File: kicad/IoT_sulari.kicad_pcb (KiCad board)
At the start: 4 copper layers, 50 x 41 mm, 44 parts, among them J1 73412-0110, J2 73412-0110, J20 694106106102, J3 20021121-00010C4LF, J4 20021121-00010C4LF, J40 693043020611, J6 20021121-00010C4LF, SW1 SW_SPST, SW2 TL3301DF160QG, SW3 TL3301DF160QG, SW4 TL3301DF160QG, SW5 TL3301DF160QG, U2 NRF9160, U20 MIC5219-3.3YM5-TR, U40 TPD3F303DPVR

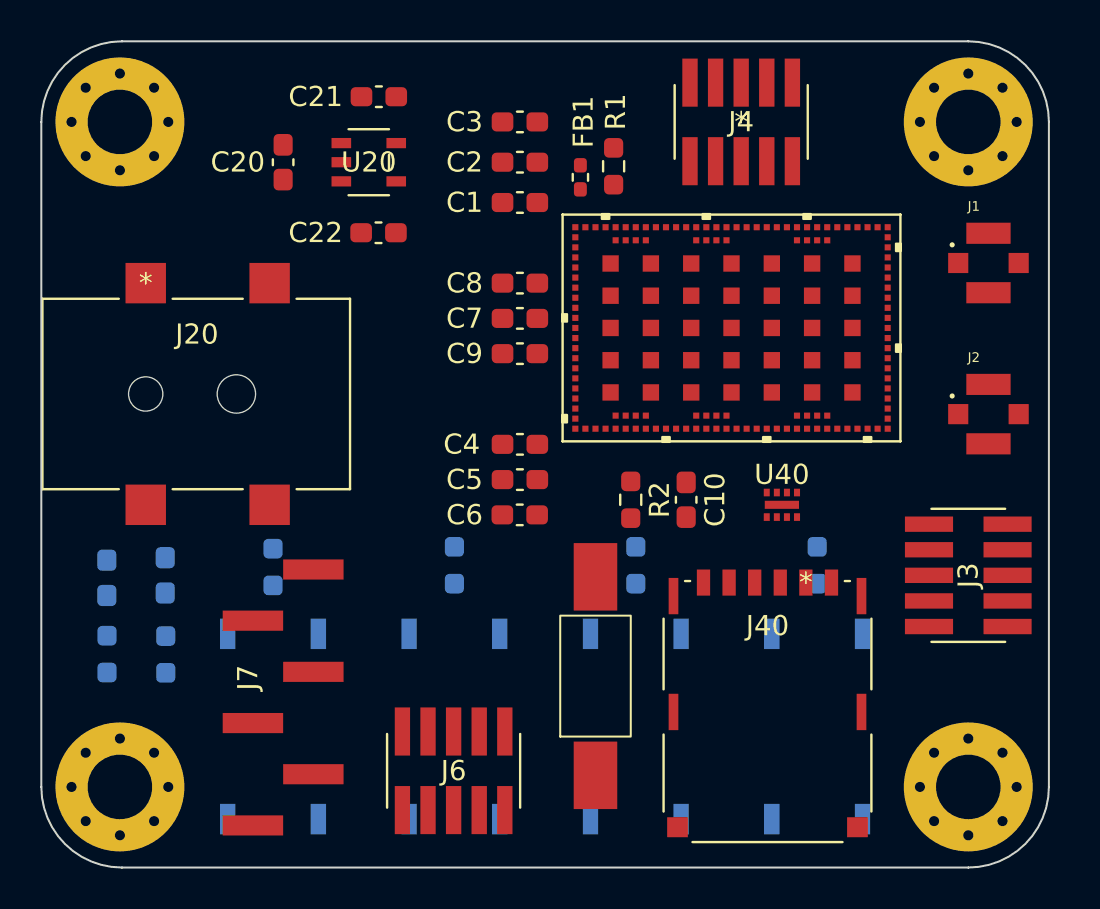
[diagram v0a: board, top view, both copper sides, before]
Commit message: routing
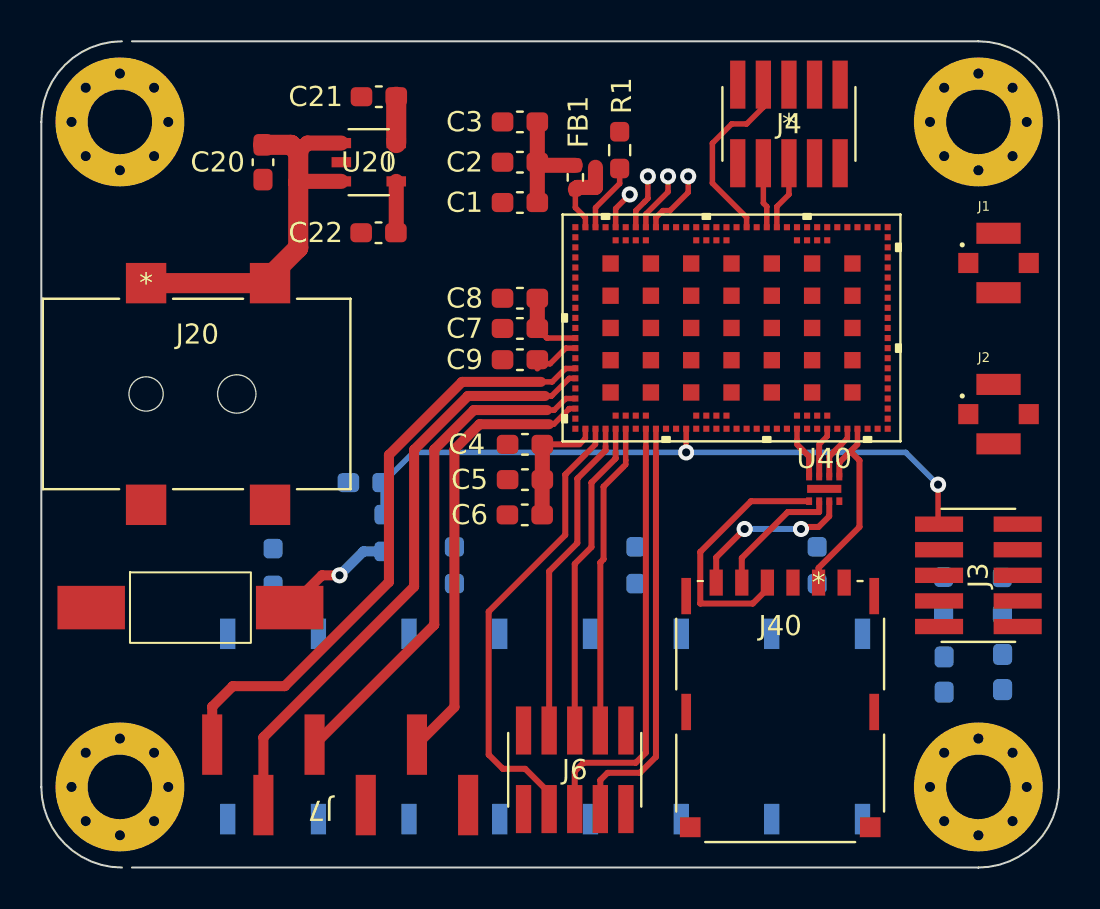
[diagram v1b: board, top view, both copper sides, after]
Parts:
- C10, R2: moved to B.Cu
- moved D2 44.7 mm to (140.2, 66.3), turned to -90 degrees
- moved R4 44.5 mm to (140.2, 62.5), turned to 90 degrees
- moved D1 39.0 mm to (137.3, 66.4), turned to -90 degrees
- moved R3 38.7 mm to (137.3, 62.5), turned to 90 degrees
- moved SW1 20.4 mm to (99.9, 63.1), turned to 0 degrees
- moved C10 15.9 mm to (108.6, 56.9), turned to 180 degrees
- moved R2 12.4 mm to (109.5, 59.4)
- moved J6 6.01 mm to (119.0, 71.2)
- moved J7 4.77 mm to (107.3, 71.4), turned to 180 degrees
- moved J4 2.37 mm to (129.6, 39.1)
- moved U40 2.24 mm to (131.4, 57.2)
- moved C20 1.00 mm to (103.5, 41.0)
- moved R1 0.85 mm to (121.2, 40.4)
- moved C8 0.75 mm to (116.2, 47.8)
- moved J40 0.63 mm to (131.1, 61.9)
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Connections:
- net /+3.3V renamed Net-(C1-Pad1)
- U2 pad 25: CS -> DC
- U2 pad 26: DC -> BUSY
- U2 pad 28: RST -> CS
- U2 pad 29: BUSY -> RST
- U2 pad 83: SDA -> TMP_ALERT
- U2 pad 84: SCL -> SDA
- U2 pad 86: TMP_ALERT -> SCL
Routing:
- net NRESET: track 0.00 -> 33.7 mm, vias 0 -> 2
- net UART_RTS: track 0.00 -> 30.6 mm
- net UART_RXD: track 0.00 -> 30.2 mm
- net UART_TXD: track 0.00 -> 25.2 mm
- net DIN: track 0.00 -> 23.0 mm
- net UART_CTS: track 0.00 -> 22.3 mm
- net CS: track 0.00 -> 21.9 mm
- net RST: track 0.00 -> 21.0 mm
- net Net-(U20-EN): track 0.00 -> 19.7 mm
- net CLK: track 0.00 -> 16.1 mm
- net DC: track 0.00 -> 15.8 mm
- net BUSY: track 0.00 -> 15.5 mm
- net Net-(U40-DATA1_OUT): track 0.00 -> 13.0 mm
- net SIM_1V8: track 0.00 -> 10.3 mm
- net SCL: track 0.00 -> 9.26 mm
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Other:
- board size 50 x 41 mm -> 50.5 x 41 mm
